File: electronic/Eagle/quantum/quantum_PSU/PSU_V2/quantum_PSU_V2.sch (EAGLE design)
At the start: 30 parts, among them J1 90814-0204, J2 90814-0204, J3 PF0030_PC, U1 7815, U2 7812, U3 7915, U4 7805, U5 LD1117AV33

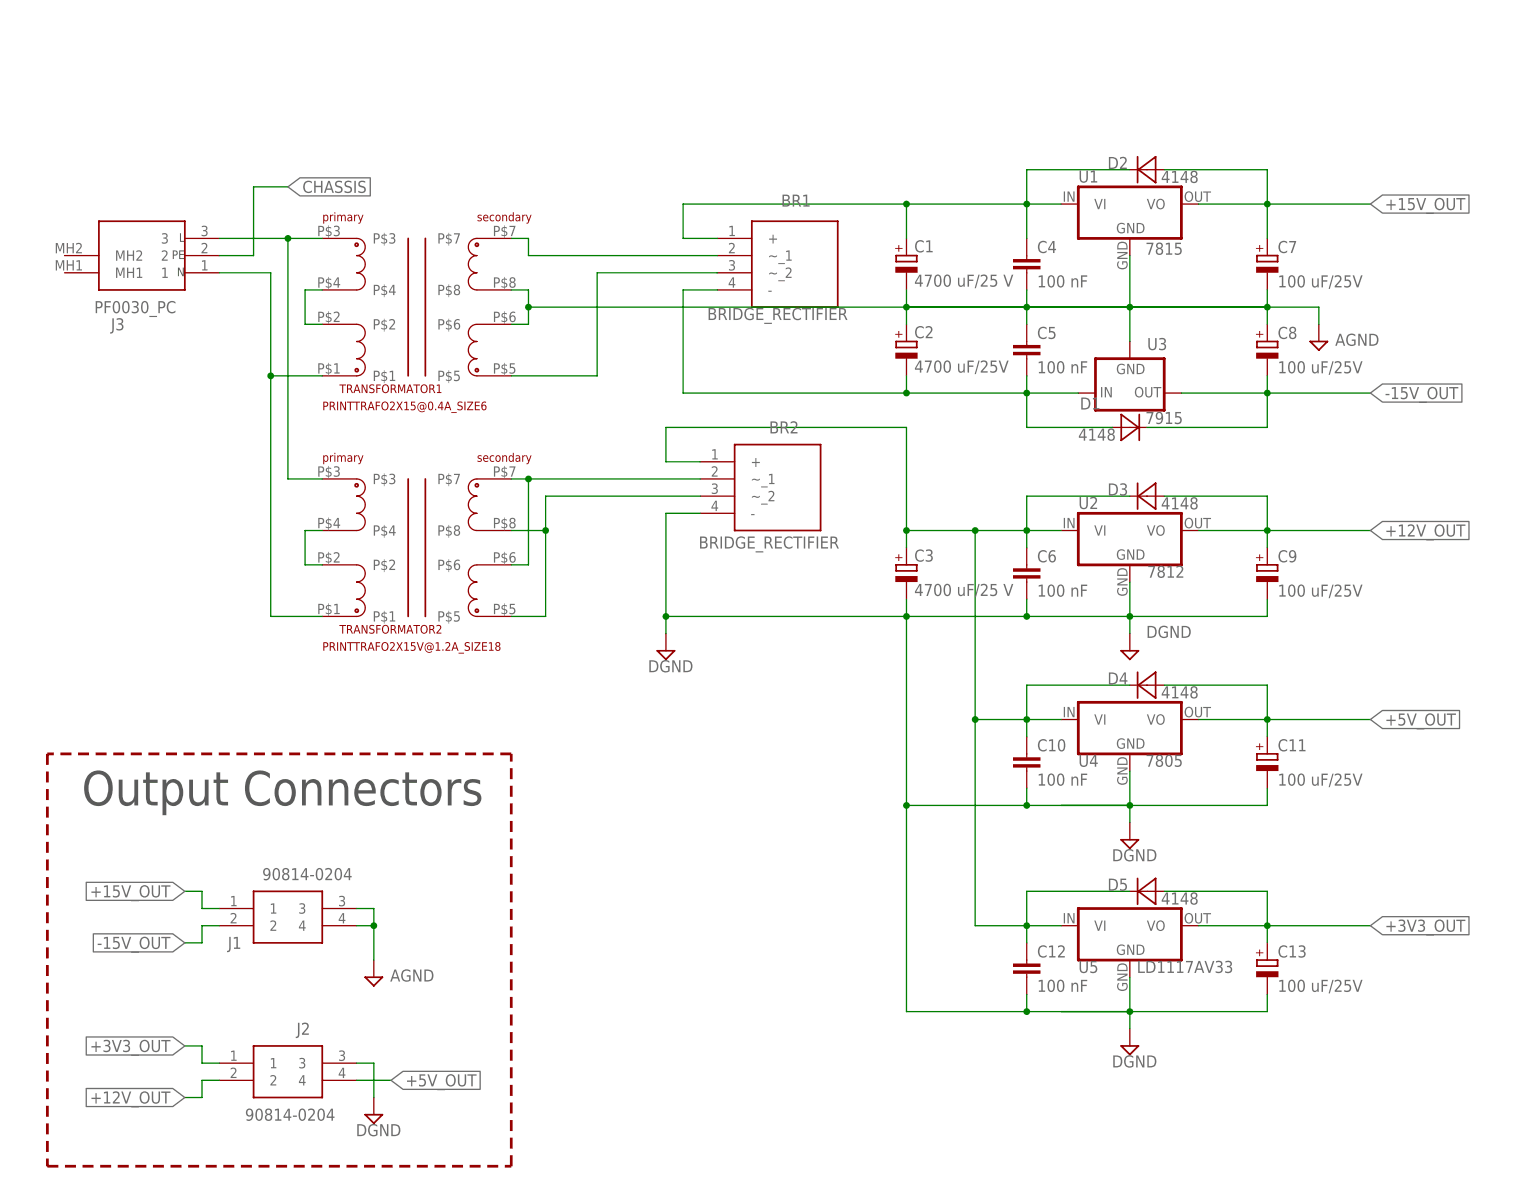
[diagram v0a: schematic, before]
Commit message: progress PSU_V2
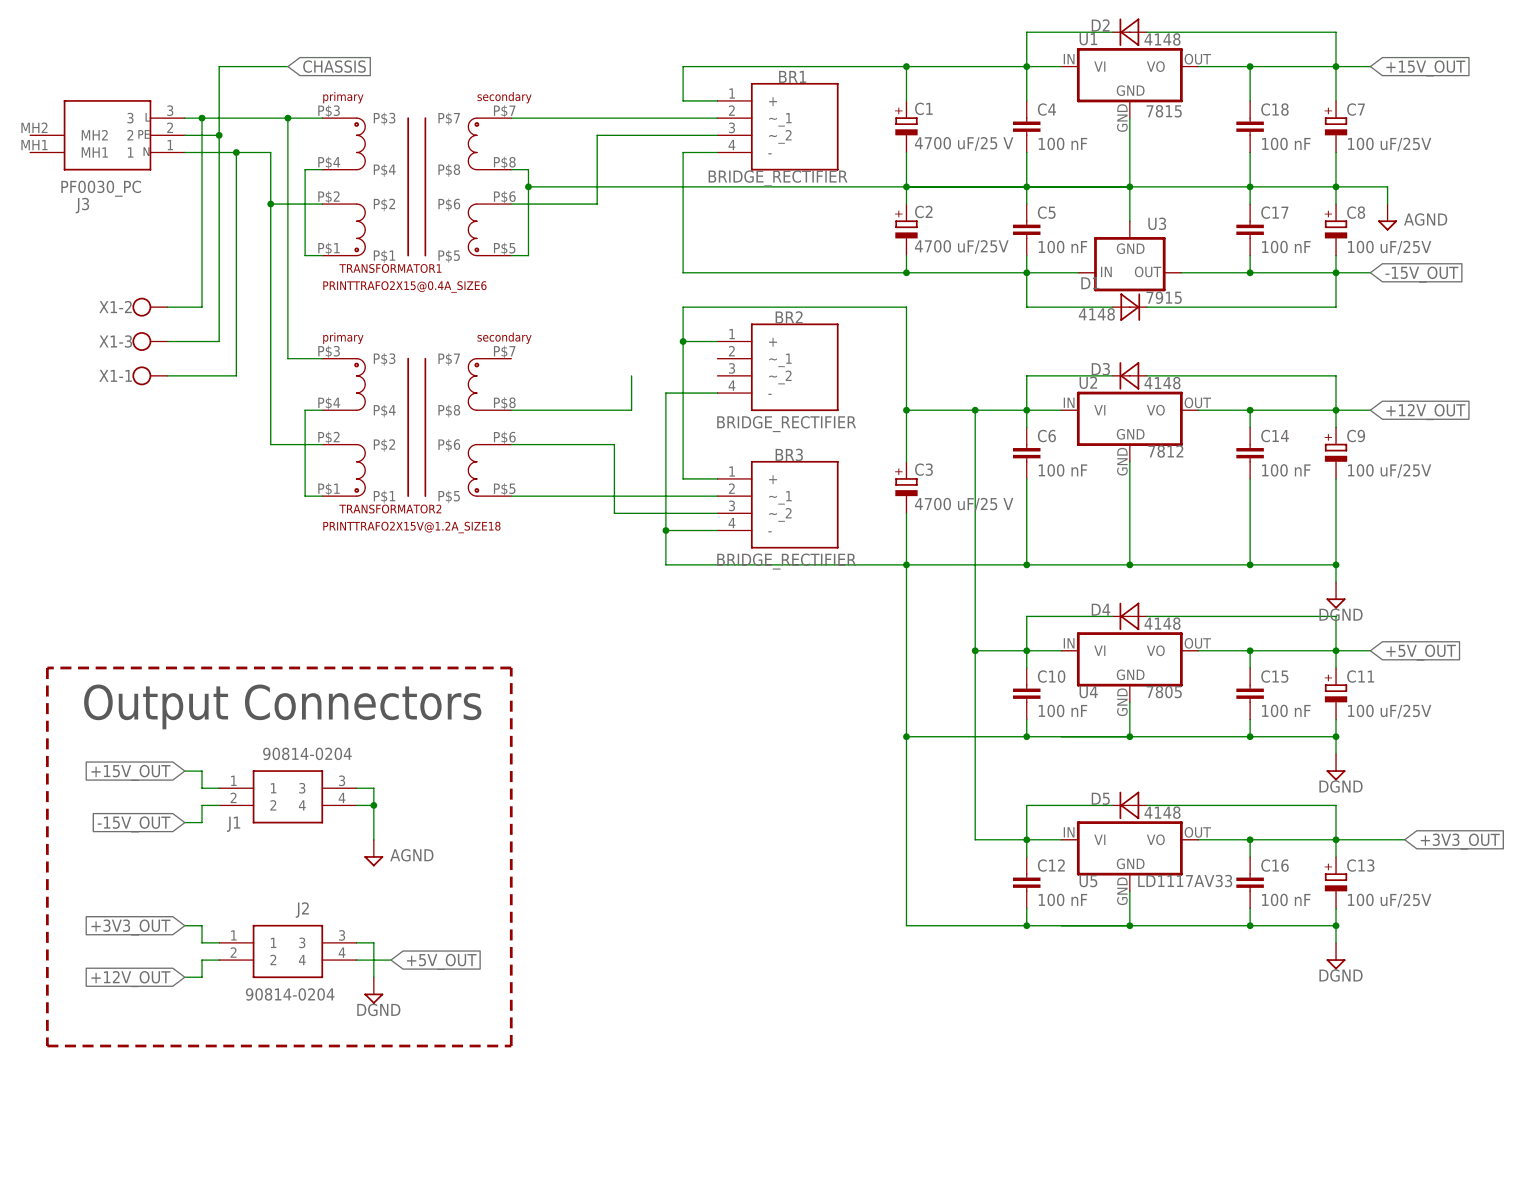
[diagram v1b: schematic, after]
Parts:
- added BR3: BRIDGE_RECTIFIER, passive components:BRIDGE_RECTIFIER
- added C14, C15, C16, C17, C18: 100 nF, passive components:CAPACITOR_5MM
- added X1: (no value), electro_mechanical:CONNECTOR_3POL
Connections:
- removed net N$1: BR2.~_1, TRANSFORMATOR2.P$6, TRANSFORMATOR2.P$7
- removed net N$13: BR1.~_2, TRANSFORMATOR1.P$5
- new net N$4: TRANSFORMATOR1.P$1, TRANSFORMATOR1.P$4
- new net N$5: TRANSFORMATOR2.P$1, TRANSFORMATOR2.P$4
- new net N$6: TRANSFORMATOR2.P$8
- net +12V_OUT: now also C14.1
- net +15V_OUT: now also C18.1
- net +3V3_OUT: now also C16.1
- net +5V_OUT: now also C15.1
- net -15V_OUT: now also C17.2
- net AGND: now also C17.1, C18.2, TRANSFORMATOR1.P$5; no longer TRANSFORMATOR1.P$6
- net CHASSIS: now also X1-3.KL
- net DGND: now also BR3.-, C14.2, C15.2, C16.2
- net N$10: now also BR3.~_1, TRANSFORMATOR2.P$5; no longer TRANSFORMATOR2.P$2, TRANSFORMATOR2.P$4
- net N$2: now also BR3.+
- net N$3: now also BR1.~_2, TRANSFORMATOR1.P$6; no longer BR2.~_2, TRANSFORMATOR2.P$5, TRANSFORMATOR2.P$8
- net N$7: now also BR3.~_2, TRANSFORMATOR2.P$6; no longer TRANSFORMATOR1.P$2, TRANSFORMATOR1.P$4
- net N$8: now also X1-2.KL
- net N$9: now also TRANSFORMATOR1.P$2, TRANSFORMATOR2.P$2, X1-1.KL; no longer TRANSFORMATOR1.P$1, TRANSFORMATOR2.P$1
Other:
- moved on the sheet: BR1, BR2, C1, C10, C11, C12, C13, C2, C3, C4, C5, C6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
